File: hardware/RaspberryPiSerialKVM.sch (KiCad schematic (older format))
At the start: 29 parts, among them J1 RASPI, J2 PC Serial Connector, K1 RM50-xx21, K2 RM50-xx21, Q1 BC548, Q2 BC548, Q3 BC548, Q4 BC559, U1 PC817, U2 PC817

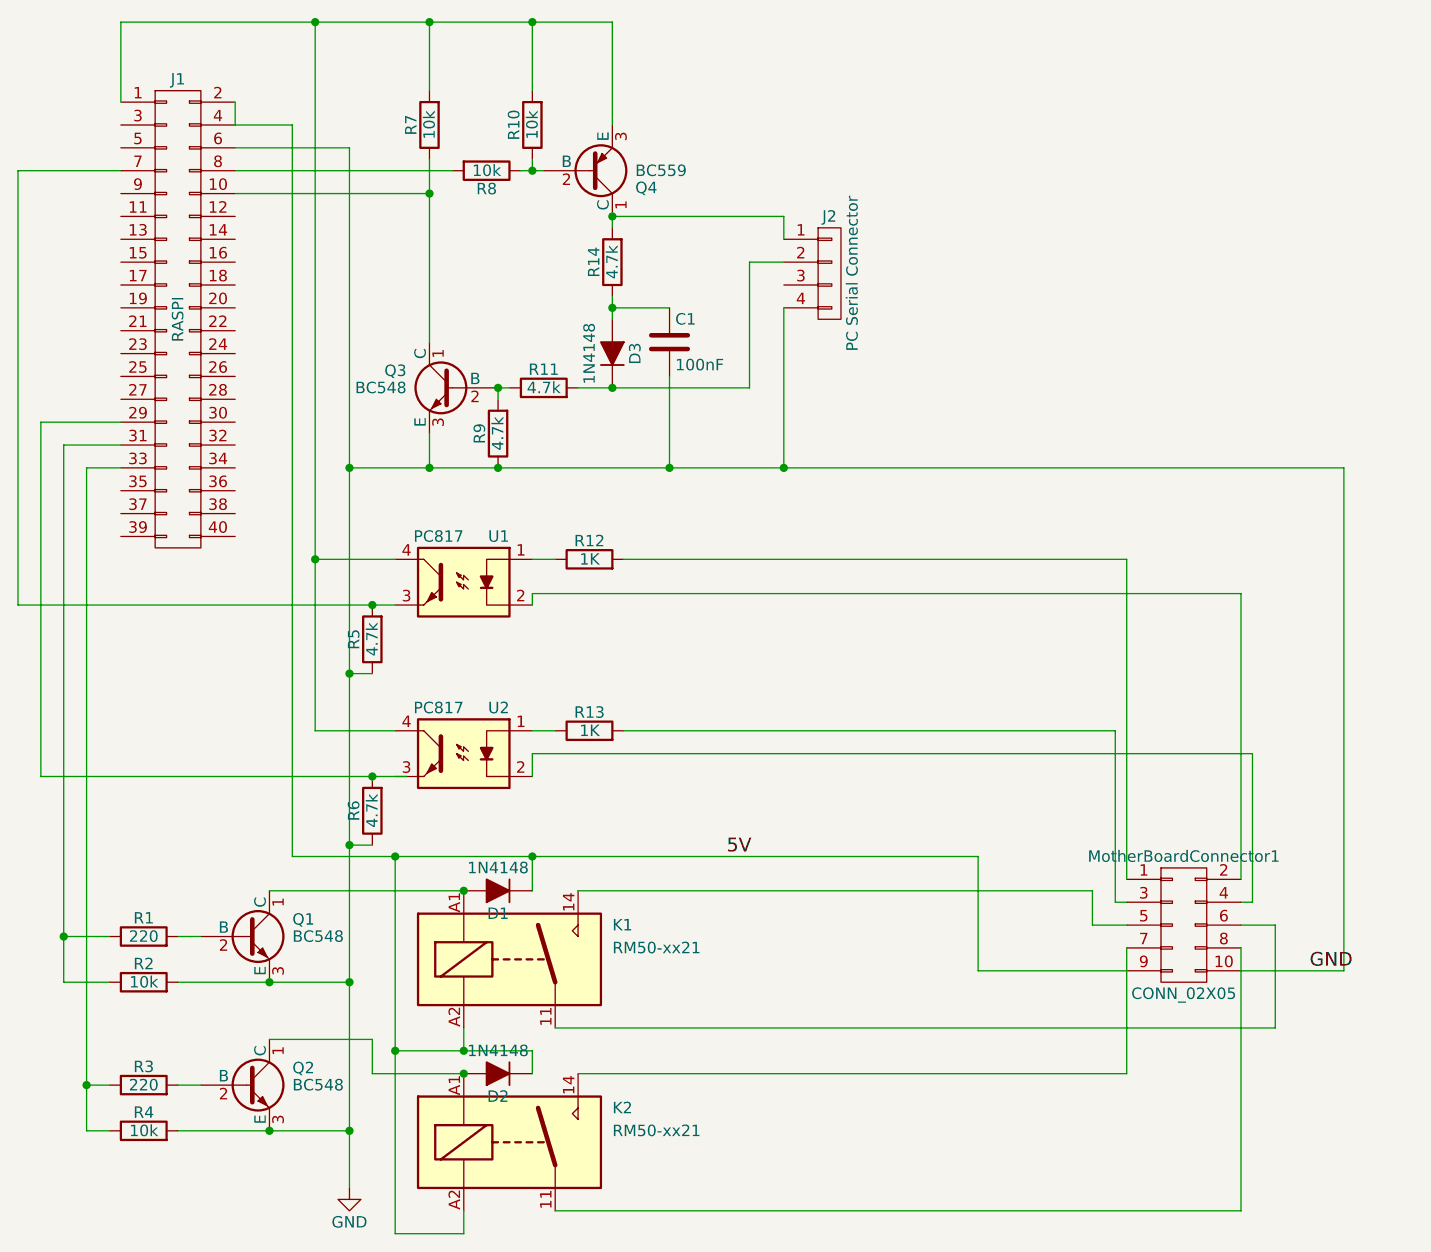
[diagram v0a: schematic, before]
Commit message: Updated Schematic
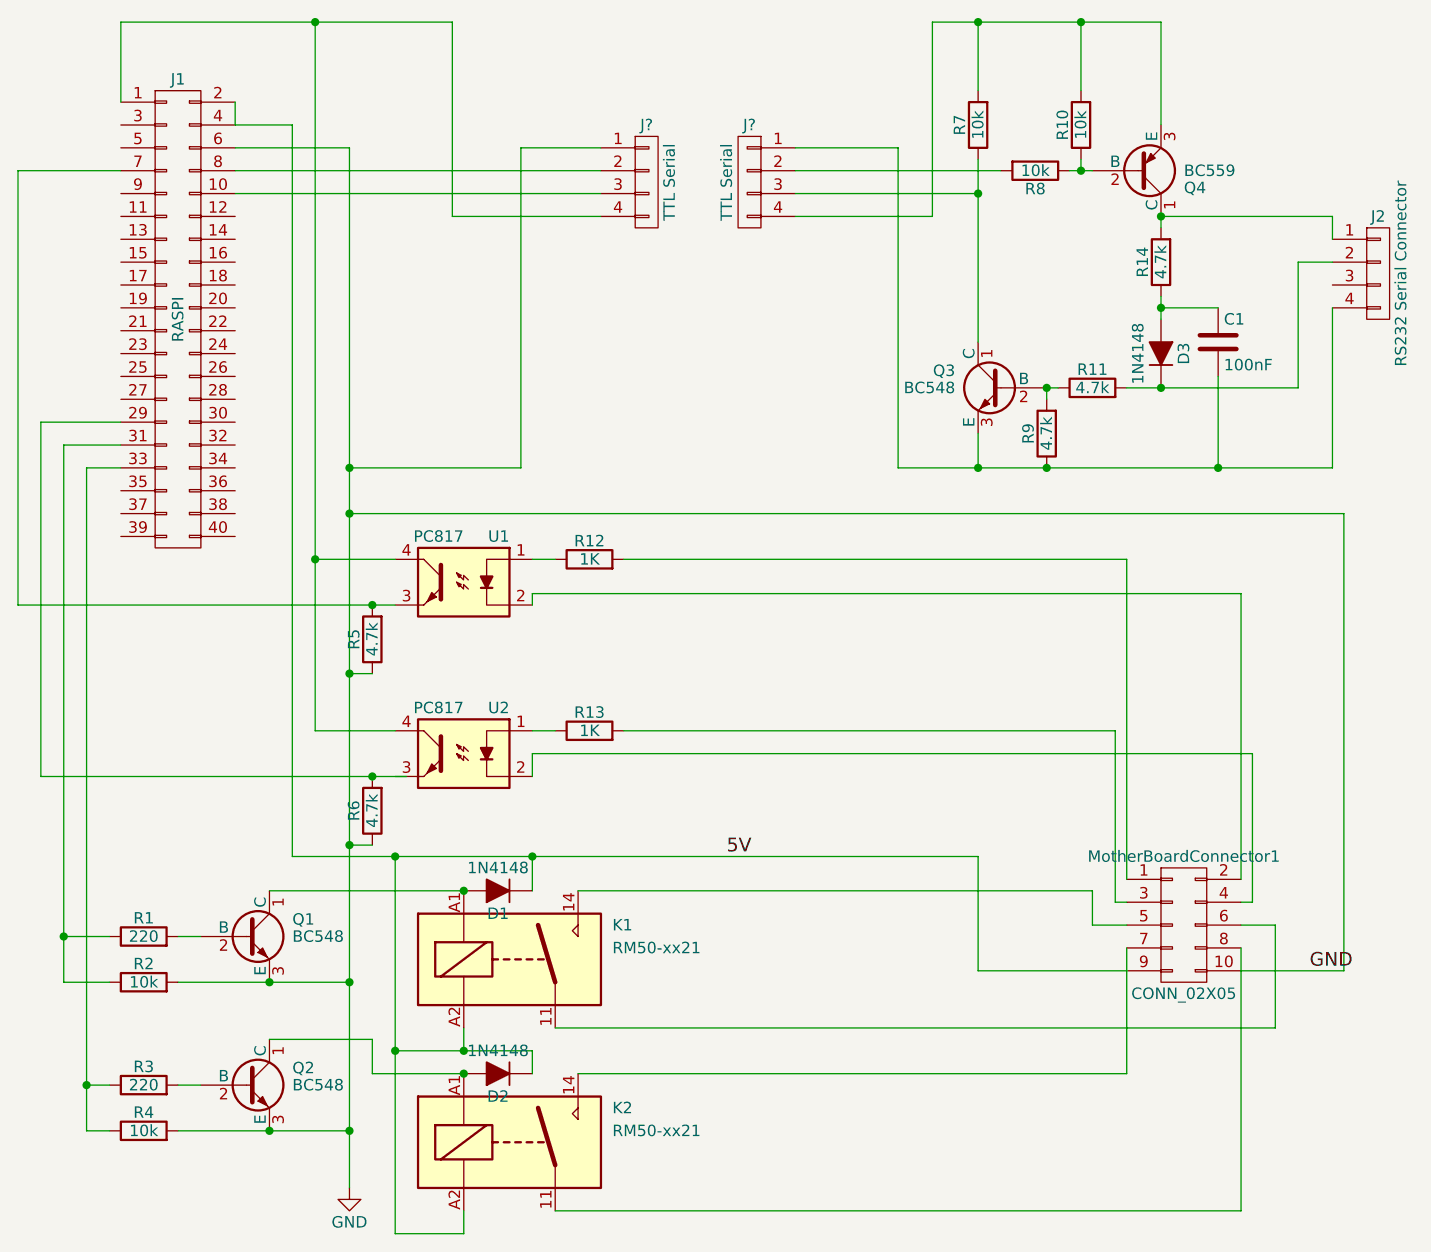
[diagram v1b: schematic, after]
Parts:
- added J? (x2): TTL Serial, symbol CONN_01X04
- J2: value PC Serial Connector -> RS232 Serial Connector
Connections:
- net GND: now also J?.1 (P1); no longer C1.2, J2.4 (P4), Q3.3 (E), R9.1
- net at J1.1 (P1), U1.4, U2.4: now also J?.4 (P4); no longer Q4.3 (E), R10.2, R7.2
- net at Q3.1 (C), R7.1: now also J?.3 (P3); no longer J1.10 (P10)
- net at J1.8 (P8): now also J?.2 (P2); no longer R8.2
- new net: J1.10 (P10), J?.3 (P3)
- new net: J?.4 (P4), Q4.3 (E), R10.2, R7.2
- new net: J?.2 (P2), R8.2
- new net: C1.2, J2.4 (P4), J?.1 (P1), Q3.3 (E), R9.1
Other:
- moved on the sheet: C1, D3, J2, Q3, Q4, R10, R11, R14, R7, R8, R9
